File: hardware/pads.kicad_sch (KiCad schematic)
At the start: 56 parts, among them J1 5V, J10 5V, J11 5V, J12 5V, J13 5V, J14 5V, J15 5V, J16 5V, J17 5V, J18 5V, J19 5V, J2 5V, J20 5V, J21 5V, J22 5V, J23 5V, J24 5V, J25 5V, J26 5V, J27 5V, J28 5V, J29 5V, J3 5V, J30 5V, J31 5V, J32 5V, J33 5V, J34 5V, J35 5V, J36 5V, J37 5V, J38 5V, J39 5V, J4 5V, J40 5V, J41 5V, J42 5V, J43 5V, J44 5V, J45 5V, J46 5V, J47 5V, J48 5V, J49 5V, J5 5V, J50 5V, J51 5V, J52 5V, J53 5V, J54 5V, J6 5V, J7 5V, J8 5V, J9 5V, P1 SM08B-SRSS-TB(LF)(SN), U8 SM06B-SRSS-TB(LF)(SN)

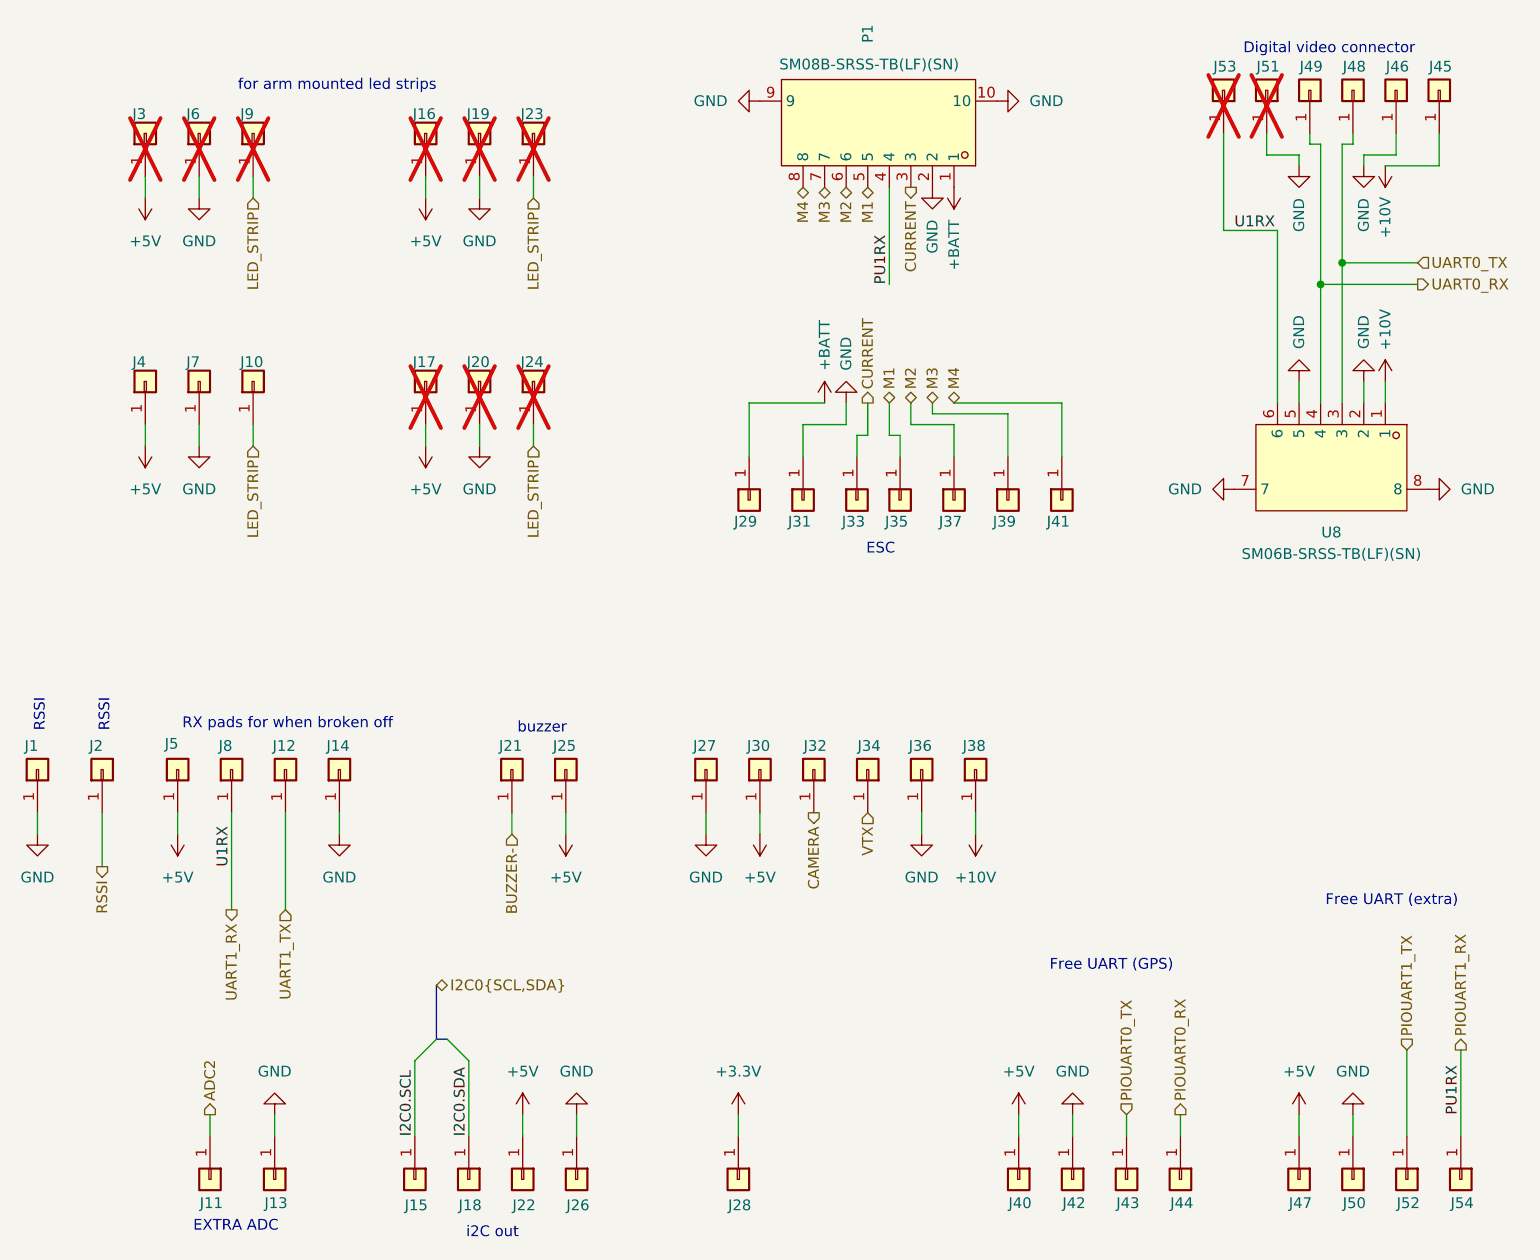
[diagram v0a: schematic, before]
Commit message: RP2354A
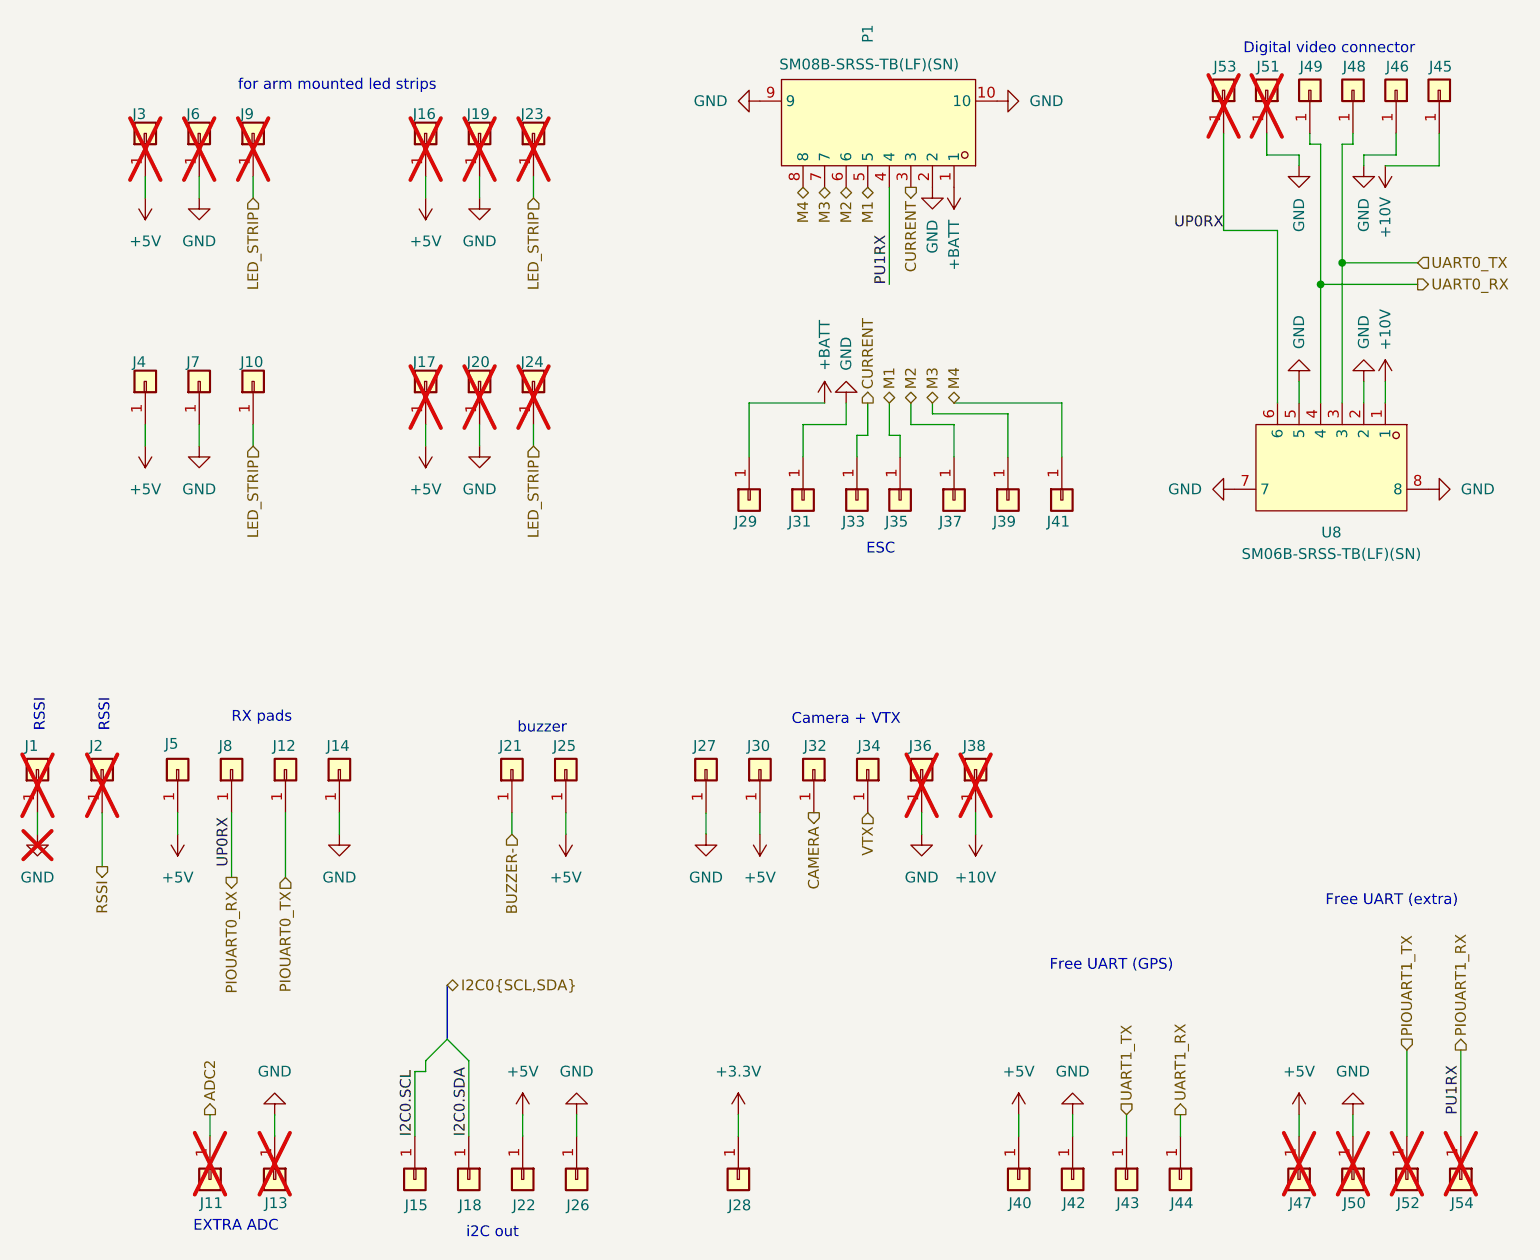
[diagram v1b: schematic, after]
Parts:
- J1, J11, J13, J2, J36, J38, J47, J50, J52, J54: now not fitted
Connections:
- net PIOUART0_RX: now also J53.1 (Pin_1), J8.1 (Pin_1), U8.6; no longer J44.1 (Pin_1)
- net PIOUART0_TX: now also J12.1 (Pin_1); no longer J43.1 (Pin_1)
- net UART1_RX: now also J44.1 (Pin_1); no longer J53.1 (Pin_1), J8.1 (Pin_1), U8.6
- net UART1_TX: now also J43.1 (Pin_1); no longer J12.1 (Pin_1)
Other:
- note added: "Camera + VTX"
- note added: "RX pads"
- note removed: "RX pads for when broken off"
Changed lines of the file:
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@@
 		)
 	)
-	(text "RX pads for when broken off"
+	(text "RX pads"
 		(exclude_from_sim no)
-		(at 62.484 97.536 0)
+		(at 59.436 96.774 0)
 		(effects
 			(font
@@
 		)
 	)
+	(text "Camera + VTX"
+		(exclude_from_sim no)
+		(at 128.27 97.028 0)
+		(effects
+			(font
+				(size 1.27 1.27)
+			)
+		)
+	)
 	(text "Digital video connector"
 		(exclude_from_sim no)
@@
 	)
 	(bus_entry
-		(at 80.01 134.62)
+		(at 81.28 134.62)
 		(size -2.54 2.54)
 		(stroke
@@
 	(wire
 		(pts
+			(xy 78.74 138.43) (xy 77.47 138.43)
+		)
+		(stroke
+			(width 0)
+			(type default)
+		)
+	)
+	(wire
+		(pts
 			(xy 111.76 107.95) (xy 111.76 110.49)
 		)
@@
 	(wire
 		(pts
+			(xy 77.47 138.43) (xy 77.47 146.05)
+		)
+		(stroke
+			(width 0)
+			(type default)
+		)
+	)
+	(wire
+		(pts
 			(xy 52.07 33.02) (xy 52.07 35.56)
 		)
@@
 	(wire
 		(pts
-			(xy 77.47 137.16) (xy 77.47 146.05)
+			(xy 78.74 137.16) (xy 78.74 138.43)
 		)
 		(stroke
@@
 	(wire
 		(pts
+			(xy 55.88 107.95) (xy 55.88 115.57)
+		)
+		(stroke
+			(width 0)
+			(type default)
+		)
+	)
+	(wire
+		(pts
 			(xy 115.57 146.05) (xy 115.57 143.51)
 		)
@@
 	(wire
 		(pts
-			(xy 62.23 107.95) (xy 62.23 119.38)
+			(xy 62.23 107.95) (xy 62.23 115.57)
 		)
 		(stroke
@@
 	(bus
 		(pts
-			(xy 80.01 128.27) (xy 80.01 134.62)
+			(xy 81.28 128.27) (xy 81.28 134.62)
 		)
 		(stroke
@@
 	(wire
 		(pts
-			(xy 55.88 107.95) (xy 55.88 119.38)
-		)
-		(stroke
-			(width 0)
-			(type default)
-		)
-	)
-	(wire
-		(pts
 			(xy 187.96 146.05) (xy 187.96 143.51)
 		)
@@
 		)
 	)
-	(bus
-		(pts
-			(xy 80.01 134.62) (xy 81.28 134.62)
-		)
-		(stroke
-			(width 0)
-			(type default)
+	(label "UP0RX"
+		(at 172.72 39.37 180)
+		(effects
+			(font
+				(size 1.27 1.27)
+			)
+			(justify right bottom)
 		)
 	)
-	(label "U1RX"
+	(label "UP0RX"
 		(at 55.88 114.3 90)
 		(effects
@@
 		)
 	)
-	(label "U1RX"
-		(at 173.99 39.37 0)
-		(effects
-			(font
-				(size 1.27 1.27)
-			)
-			(justify left bottom)
-		)
-	)
 	(label "PU1RX"
 		(at 200.66 143.51 90)
@@
 		)
 	)
-	(hierarchical_label "PIOUART0_RX"
-		(shape output)
-		(at 167.64 143.51 90)
-		(effects
-			(font
-				(size 1.27 1.27)
-			)
-			(justify left)
-		)
-	)
 	(hierarchical_label "CAMERA"
 		(shape output)
@@
 	(hierarchical_label "PIOUART0_TX"
 		(shape input)
-		(at 161.29 143.51 90)
+		(at 62.23 115.57 270)
 		(effects
 			(font
 				(size 1.27 1.27)
 			)
-			(justify left)
+			(justify right)
 		)
 	)
@@
 	(hierarchical_label "I2C0{SCL,SDA}"
 		(shape bidirectional)
-		(at 80.01 128.27 0)
+		(at 81.28 128.27 0)
 		(effects
 			(font
@@
 		)
 	)
+	(hierarchical_label "PIOUART0_RX"
+		(shape output)
+		(at 55.88 115.57 270)
+		(effects
+			(font
+				(size 1.27 1.27)
+			)
+			(justify right)
+		)
+	)
 	(hierarchical_label "M1"
 		(shape bidirectional)
@@
 		)
 	)
-	(hierarchical_label "CURRENT"
+	(hierarchical_label "UART1_RX"
 		(shape output)
-		(at 130.81 59.69 90)
+		(at 167.64 143.51 90)
 		(effects
 			(font
@@
 		)
 	)
-	(hierarchical_label "RSSI"
+	(hierarchical_label "CURRENT"
 		(shape output)
-		(at 40.64 114.3 270)
+		(at 130.81 59.69 90)
 		(effects
 			(font
 				(size 1.27 1.27)
 			)
-			(justify right)
+			(justify left)
 		)
 	)
-	(hierarchical_label "UART1_RX"
+	(hierarchical_label "RSSI"
 		(shape output)
-		(at 55.88 119.38 270)
+		(at 40.64 114.3 270)
 		(effects
 			(font
@@
 		)
 	)
-	(hierarchical_label "UART1_TX"
-		(shape input)
-		(at 62.23 119.38 270)
-		(effects
-			(font
-				(size 1.27 1.27)
-			)
-			(justify right)
-		)
-	)
 	(hierarchical_label "PIOUART1_RX"
 		(shape output)
@@
 		)
 	)
+	(hierarchical_label "UART1_TX"
+		(shape input)
+		(at 161.29 143.51 90)
+		(effects
+			(font
+				(size 1.27 1.27)
+			)
+			(justify left)
+		)
+	)
 	(hierarchical_label "VTX"
 		(shape input)
@@
 		(exclude_from_sim no)
 		(in_bom no)
-		(on_board yes)
+		(on_board no)
 		(in_pos_files yes)
-		(dnp no)
+		(dnp yes)
 		(property "Reference" "J50"
 			(at 189.484 153.924 90)
@@
 		(exclude_from_sim no)
 		(in_bom no)
-		(on_board yes)
+		(on_board no)
 		(in_pos_files yes)
-		(dnp no)
+		(dnp yes)
 		(fields_autoplaced yes)
 		(property "Reference" "#PWR087"
@@
 		(exclude_from_sim no)
 		(in_bom no)
-		(on_board yes)
+		(on_board no)
 		(in_pos_files yes)
-		(dnp no)
+		(dnp yes)
 		(property "Reference" "J36"
 			(at 135.636 100.076 90)
@@
 		(exclude_from_sim no)
 		(in_bom no)
-		(on_board yes)
+		(on_board no)
 		(in_pos_files yes)
-		(dnp no)
+		(dnp yes)
 		(property "Reference" "J38"
 			(at 141.986 100.076 90)
@@
 		(exclude_from_sim no)
 		(in_bom no)
-		(on_board yes)
+		(on_board no)
 		(in_pos_files yes)
-		(dnp no)
+		(dnp yes)
 		(property "Reference" "J1"
 			(at 31.496 100.076 90)
@@
 		(exclude_from_sim no)
 		(in_bom no)
-		(on_board yes)
+		(on_board no)
 		(in_pos_files yes)
-		(dnp no)
+		(dnp yes)
 		(property "Reference" "J13"
 			(at 62.484 153.924 90)
@@
 		(exclude_from_sim no)
 		(in_bom no)
-		(on_board yes)
+		(on_board no)
 		(in_pos_files yes)
-		(dnp no)
+		(dnp yes)
 		(property "Reference" "J2"
 			(at 39.116 100.076 90)
@@
 		(exclude_from_sim no)
 		(in_bom no)
-		(on_board yes)
+		(on_board no)
 		(in_pos_files yes)
-		(dnp no)
+		(dnp yes)
 		(property "Reference" "J54"
 			(at 202.184 153.924 90)
@@
 		(exclude_from_sim no)
 		(in_bom no)
-		(on_board yes)
+		(on_board no)
 		(in_pos_files yes)
-		(dnp no)
+		(dnp yes)
 		(property "Reference" "J11"
 			(at 54.864 153.924 90)
@@
 		(exclude_from_sim no)
 		(in_bom no)
-		(on_board yes)
+		(on_board no)
 		(in_pos_files yes)
-		(dnp no)
+		(dnp yes)
 		(property "Reference" "J47"
 			(at 183.134 153.924 90)
@@
 		(exclude_from_sim no)
 		(in_bom no)
-		(on_board yes)
+		(on_board no)
 		(in_pos_files yes)
-		(dnp no)
+		(dnp yes)
 		(property "Reference" "J52"
 			(at 195.834 153.924 90)
